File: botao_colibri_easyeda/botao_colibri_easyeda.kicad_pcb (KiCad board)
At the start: 2 copper layers, 72.5 x 47.1 mm, 6 parts

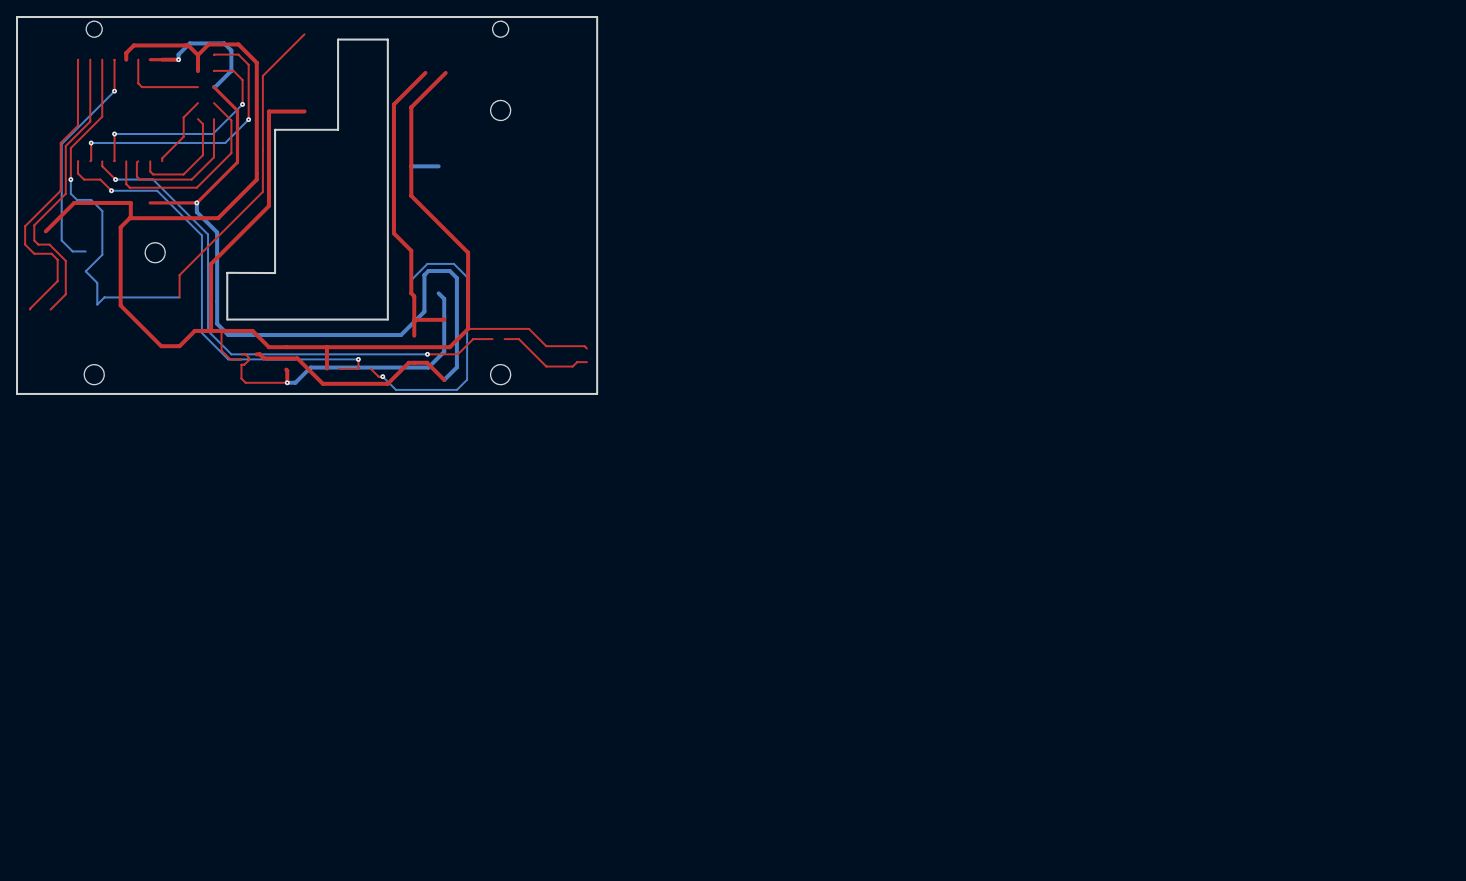
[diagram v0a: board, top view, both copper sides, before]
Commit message: LImpeza board placa botão
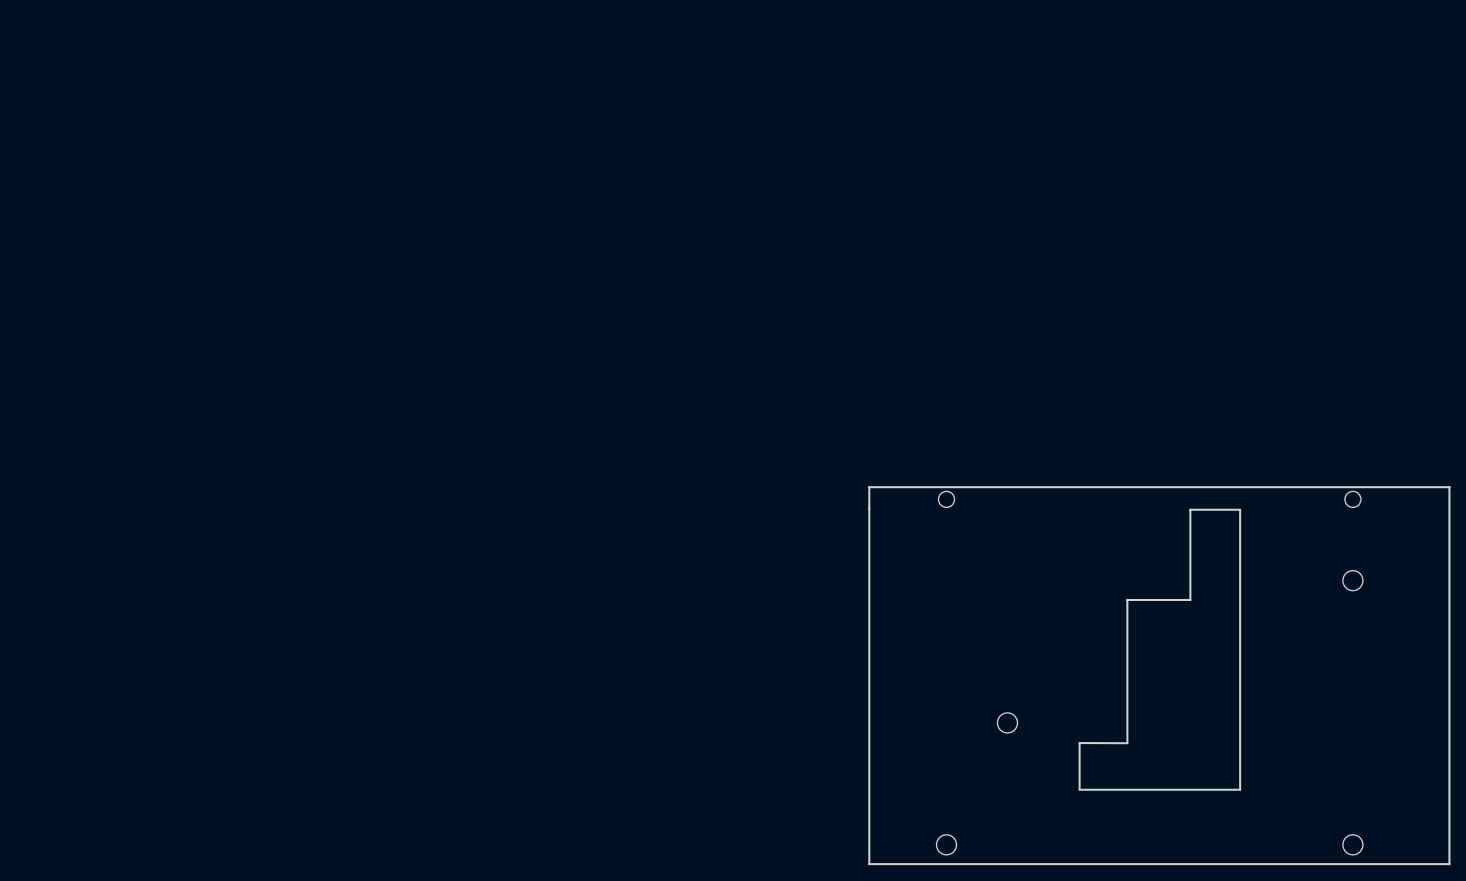
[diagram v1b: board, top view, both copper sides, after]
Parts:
- moved H1 121.7 mm to (167.0, 70.5)
- moved H2 121.7 mm to (116.2, 103.5)
- moved H3 121.7 mm to (167.0, 103.5)
- moved H4 121.7 mm to (123.8, 88.2)
- moved H5 121.7 mm to (116.2, 60.3)
- moved H6 121.7 mm to (167.0, 60.3)
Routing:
- net 0: track 947.7 -> 0.00 mm, vias 14 -> 0
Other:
- board text removed: "4.5 AUDIO-TH_PJ307C"
- board text removed: "4.5 C1206"
- board text removed: "4.5 CONN-TH_10P-P2.00_PHD2.0MM-2X5"
- board text removed: "4.5 DIODE"
- board text removed: "4.5 HDR-F-2.54_1X2"
- board text removed: "4.5 HDR-M-2.54_1X1"
- board text removed: "4.5 HM-11"
- board text removed: "4.5 LED 5MM"
- board text removed: "4.5 LED0603_RED"
- board text removed: "4.5 MIC5365-3.3YC5-TR 3.3V REGULATOR"
- board text removed: "4.5 R0603"
- board text removed: "4.5 SOD-123_L2.8-W1.8-LS3.7-RD"
- board text removed: "4.5 TP4056"
- board text removed: "5.5118"
